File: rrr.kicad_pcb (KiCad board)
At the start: 2 copper layers, 24 x 12 mm, 8 parts, among them J1 Conn_01x01_Male, J2 Conn_01x01_Male, J3 Conn_01x01_Male, J4 Conn_01x01_Male, J5 Conn_01x01_Male, J6 Conn_01x01_Male, K1 SILxx-1Axx-71x, K2 SILxx-1Axx-71x

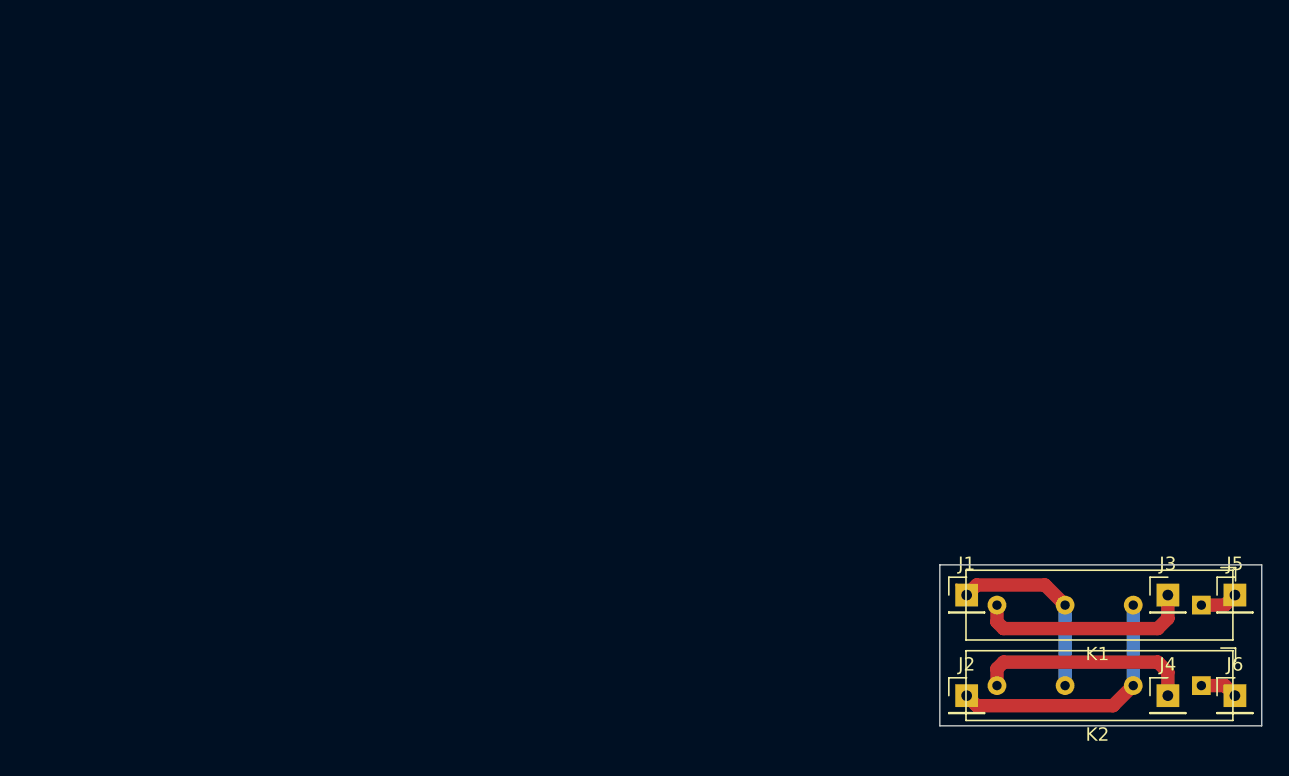
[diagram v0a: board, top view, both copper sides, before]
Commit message: Initial commit for 25065637
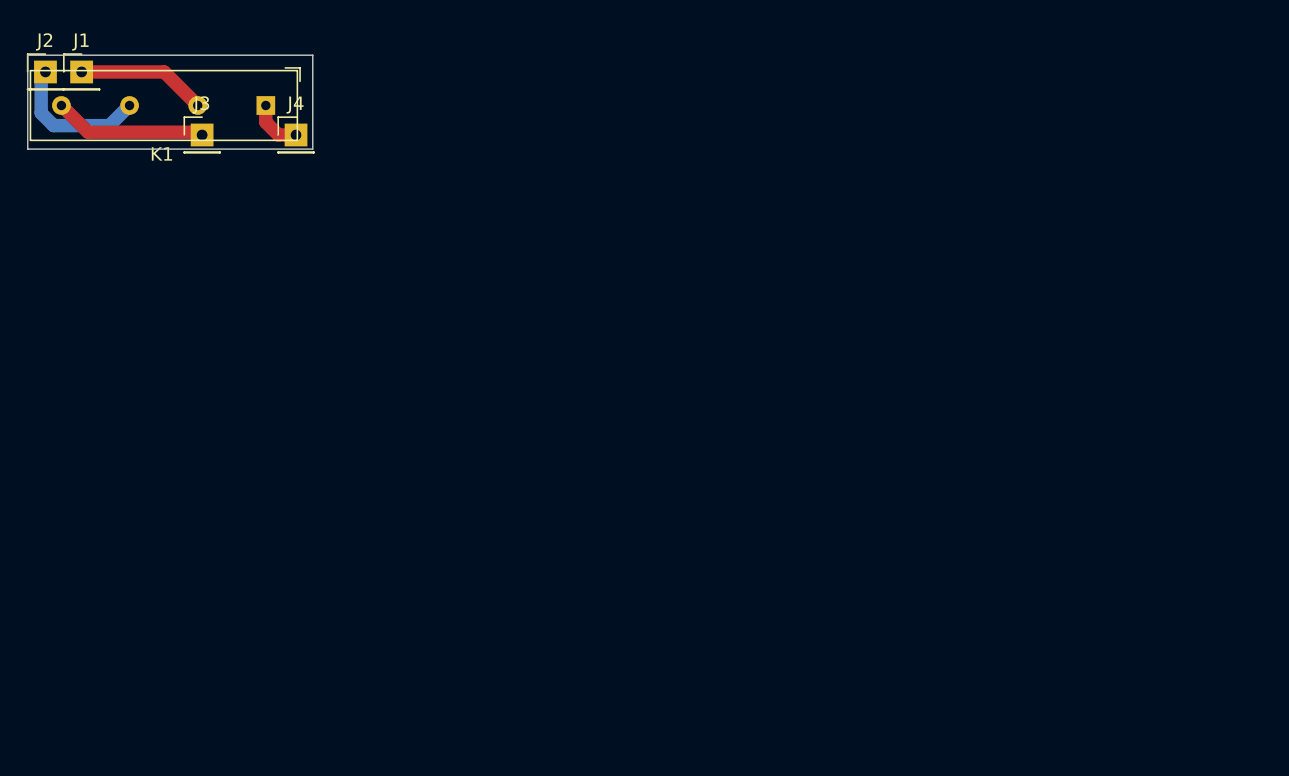
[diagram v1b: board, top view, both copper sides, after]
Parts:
- removed J5, J6: Conn_01x01_Male, Connector_PinHeader_2.54mm:PinHeader_1x01_P2.54mm_Vertical
- removed K2: SILxx-1Axx-71x, Relay_THT:Relay_SPST_StandexMeder_SIL_Form1A
- moved J1 80.7 mm to (16.0, 13.2)
- moved J3 79.8 mm to (25.0, 17.9)
- moved K1 79.1 mm to (29.8, 15.8)
- moved J2 79.0 mm to (13.3, 13.2)
- moved J4 77.3 mm to (32.0, 17.9)
- renumbered J2 to J1, J1 to J2
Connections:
- K1 pad 1: Net-(J5-Pad1) -> Net-(J4-Pad1)
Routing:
- net Net-(J4-Pad1): track 16.3 -> 3.89 mm
- net Net-(J1-Pad1): track 19.4 -> 9.69 mm
- net Net-(J3-Pad1): track 16.3 -> 11.4 mm
- net Net-(J2-Pad1): track 15.3 -> 10.8 mm
- net Net-(J6-Pad1): track 2.81 -> 0.00 mm
- net Net-(J5-Pad1): track 2.81 -> 0.00 mm
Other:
- board size 24 x 12 mm -> 21.2 x 7 mm
- board text removed: "relay reed replacement"
